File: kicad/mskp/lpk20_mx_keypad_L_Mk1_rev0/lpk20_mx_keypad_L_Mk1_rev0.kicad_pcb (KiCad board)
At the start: 2 copper layers, 122 x 97 mm, 25 parts, among them J1 Conn_01x12_Socket, SW1 Switch, SW10 Switch, SW2 Switch, SW3 Switch, SW4 Switch, SW5 Switch, SW6 Switch, SW7 Switch, SW8 Switch, SW9 Switch

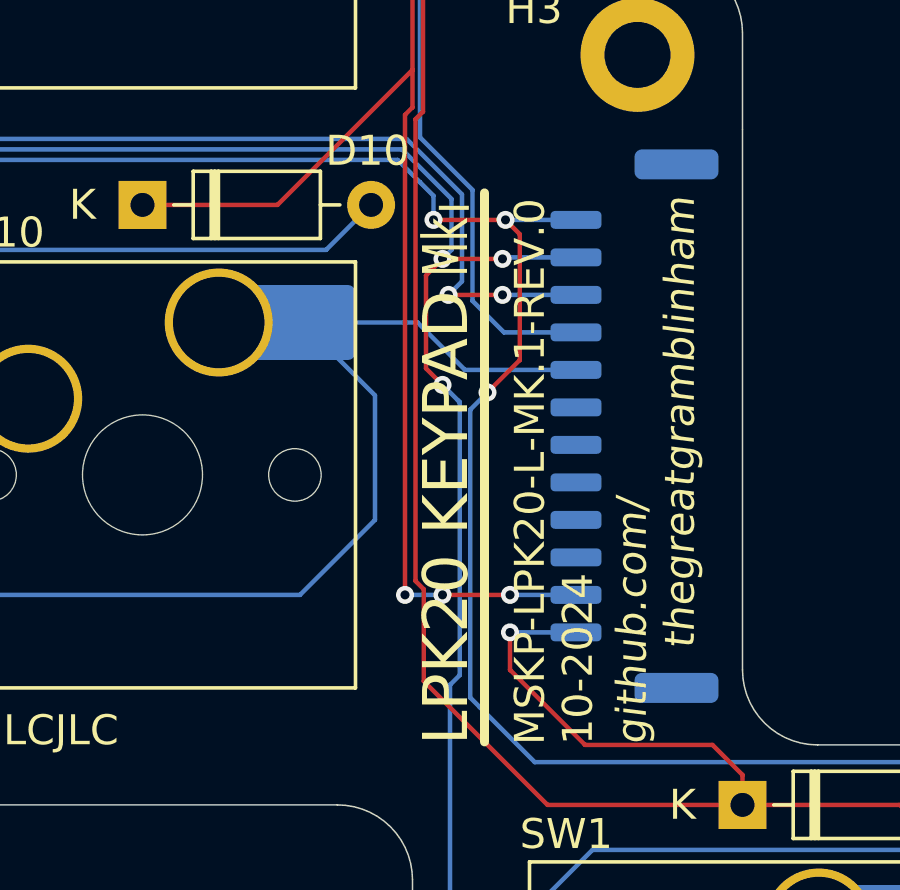
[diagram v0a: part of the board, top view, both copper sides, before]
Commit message: Final tweaks to PCBs before second round of mskp fabrications
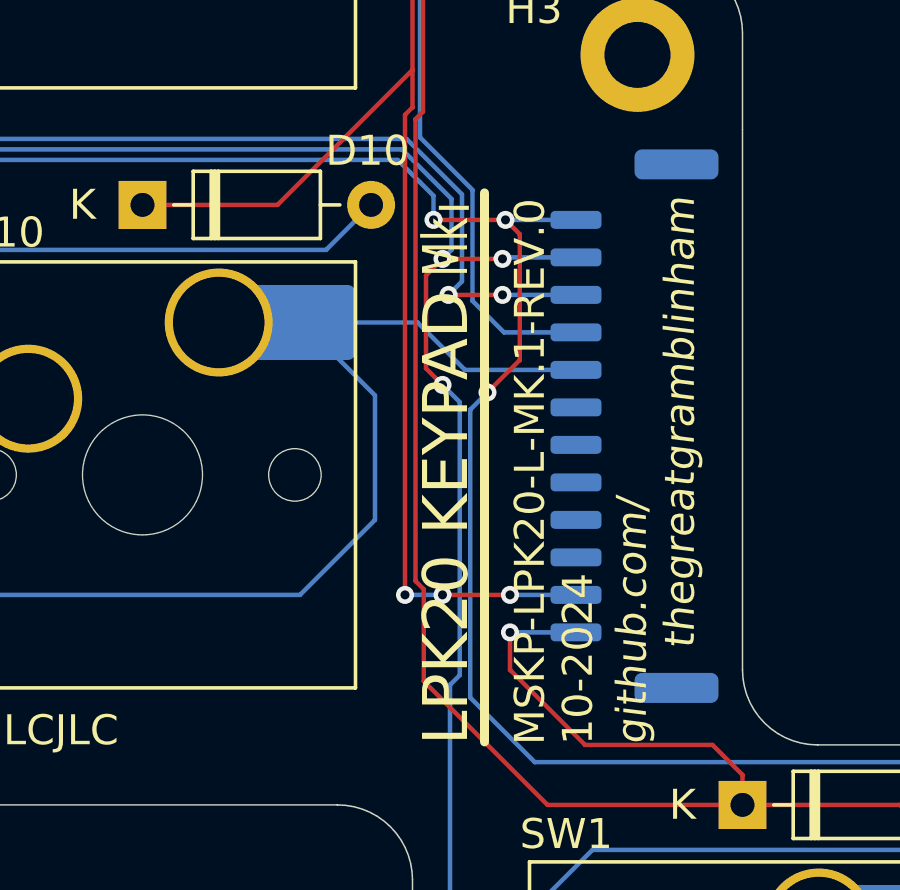
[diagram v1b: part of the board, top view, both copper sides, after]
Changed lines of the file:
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@@
 			(plot_on_all_layers_selection 0x0000000_00000000)
 			(disableapertmacros no)
-			(usegerberextensions no)
-			(usegerberattributes yes)
-			(usegerberadvancedattributes yes)
-			(creategerberjobfile yes)
+			(usegerberextensions yes)
+			(usegerberattributes no)
+			(usegerberadvancedattributes no)
+			(creategerberjobfile no)
 			(dashed_line_dash_ratio 12.000000)
 			(dashed_line_gap_ratio 3.000000)
 			(svgprecision 4)
 			(plotframeref no)
-			(viasonmask no)
+			(viasonmask yes)
 			(mode 1)
 			(useauxorigin no)
@@
 			(psa4output no)
 			(plotreference yes)
-			(plotvalue yes)
+			(plotvalue no)
 			(plotfptext yes)
 			(plotinvisibletext no)
 			(sketchpadsonfab no)
-			(subtractmaskfromsilk no)
+			(subtractmaskfromsilk yes)
 			(outputformat 1)
 			(mirror no)
-			(drillshape 1)
+			(drillshape 0)
 			(scaleselection 1)
-			(outputdirectory "")
+			(outputdirectory "lpk20_l_mk1_exports")
 		)
 	)
@@
 	)
 	(segment
-		(start 143.249999 98.75)
-		(end 143.228975 98.728976)
-		(width 0.15)
-		(layer "B.Cu")
-		(net 17)
-	)
-	(segment
 		(start 145.074999 100.575)
 		(end 143.249999 98.75)
@@
 	)
 	(segment
-		(start 141.25 81.244974)
-		(end 141.25 81.25)
-		(width 0.15)
-		(layer "B.Cu")
-		(net 17)
-	)
-	(segment
 		(start 122.6 79.1)
 		(end 124 80.5)
@@
 		(width 0.15)
 		(layer "B.Cu")
-		(net 18)
-	)
-	(segment
-		(start 142.575 88.575)
-		(end 142.5 88.5)
-		(width 0.15)
-		(layer "B.Cu")
